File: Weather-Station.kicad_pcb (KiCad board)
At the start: 2 copper layers, 100 x 100 mm, 69 parts, among them J1 PV IN, J10 Lightning Sensor, J11 RG-15 Rain Sensor, J12 BME280 Sensor, J2 TX1, J3 TX2, J4 RX1, J5 RX2, J6 RTD1, J7 RTD2, J8 PDB-C139, J9 TMP36GT9Z, U1 MCP73812T-420I-OT, U2 TPS3700DDCR, U3 TDC1000PW, U4 SiT8918AE-13-33E-5.000000G, U5 TPS73633DBV, U6 TDC7200PW, U7 Wemos_S2, U8 ADS1115IDGS

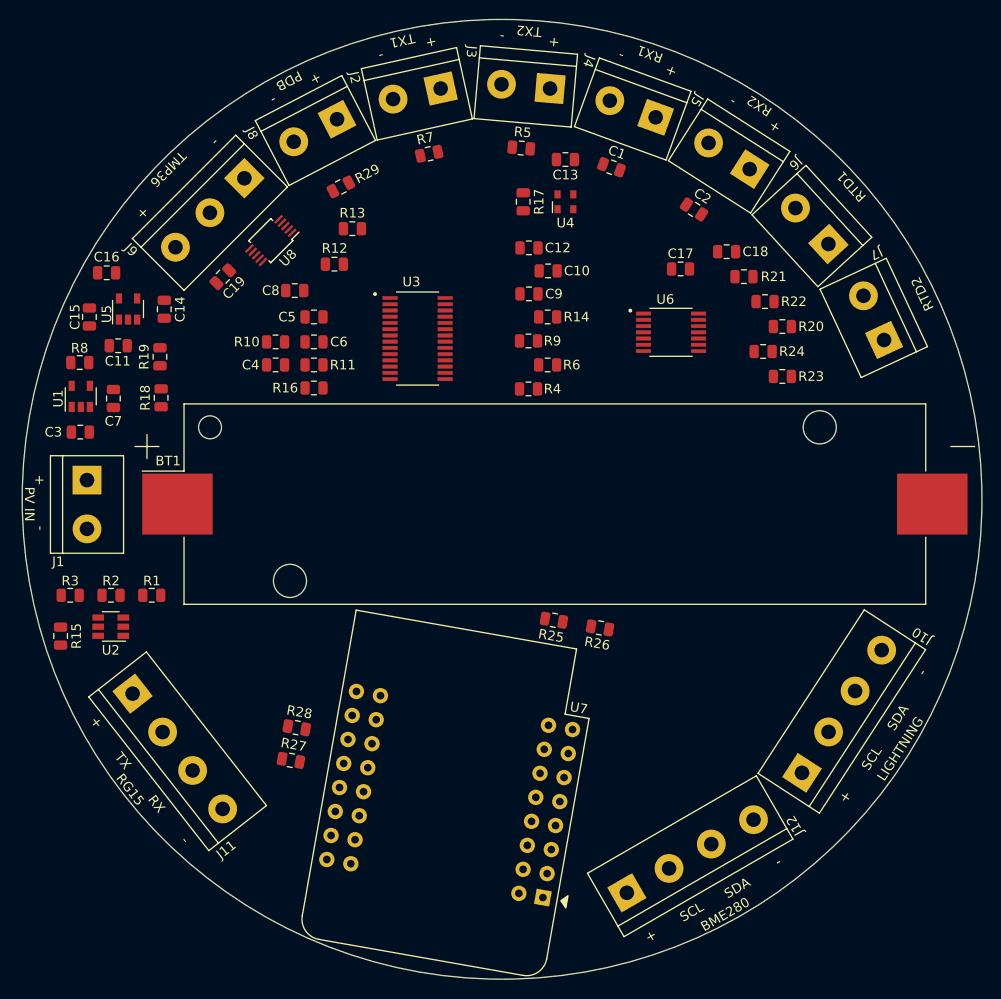
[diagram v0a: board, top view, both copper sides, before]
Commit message: to be continued
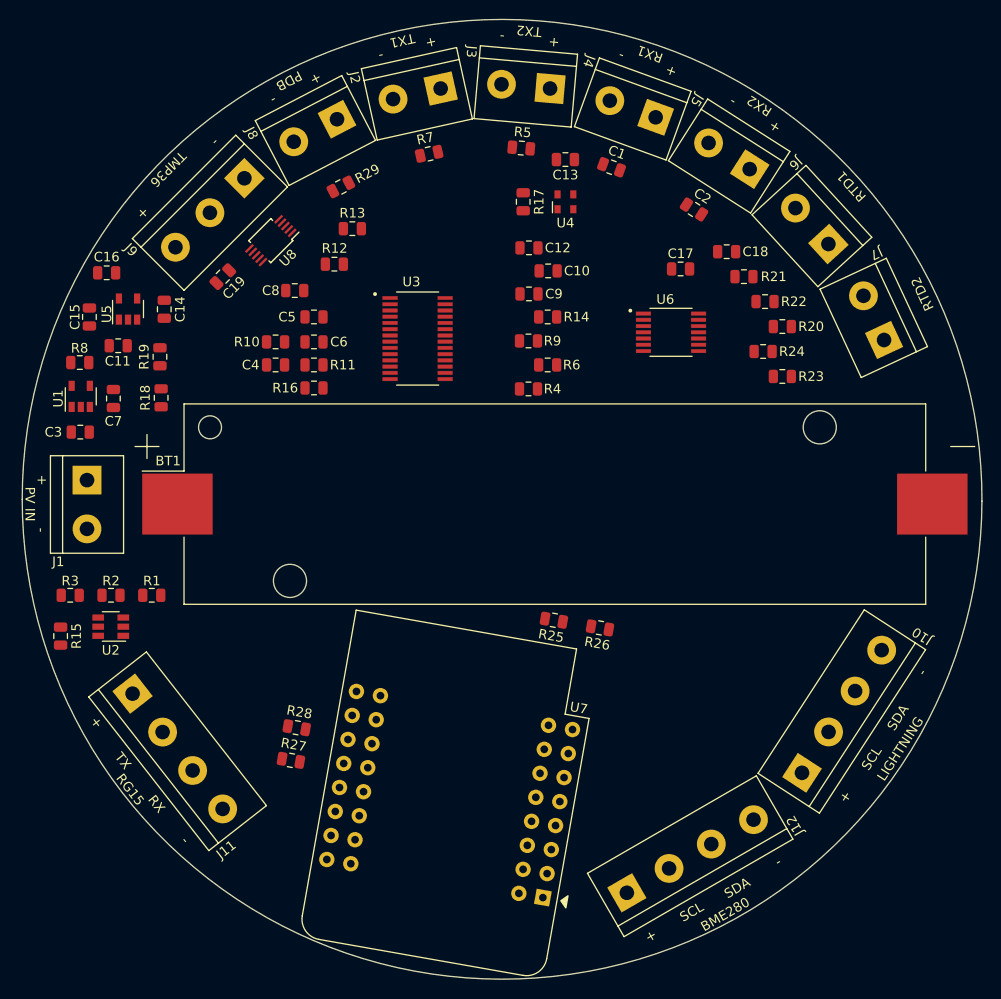
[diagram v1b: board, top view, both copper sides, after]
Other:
- outline, holes or cut-outs redrawn
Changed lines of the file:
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@@
   (general
     (thickness 1.6)
-    (drawings 39)
+    (drawings 40)
     (tracks 0)
     (zones 0)
@@
     )
   )
+  (gr_arc (start 103 94) (end 152.999599 94.199997) (angle -180.2291814) (layer Edge.Cuts) (width 0.05))
+  (gr_arc (start 103 94) (end 53 94) (angle -179.7708181) (layer Edge.Cuts) (width 0.05))
   (gr_text RTD2 (at 146.8 72.6 115) (layer F.SilkS)
     (effects (font (size 1 1) (thickness 0.15)))
@@
     (effects (font (size 1 1) (thickness 0.15)))
   )
-  (gr_text "PV IN" (at 53.75 94.5 270) (layer F.SilkS)
-    (effects (font (size 1 1) (thickness 0.15)))
-  )
-  (gr_text - (at 54.75 97 90) (layer F.SilkS)
-    (effects (font (size 1 1) (thickness 0.15)))
-  )
-  (gr_text + (at 54.75 92 90) (layer F.SilkS)
-    (effects (font (size 1 1) (thickness 0.15)))
-  )
-  (gr_circle (center 103 94) (end 153 94) (layer Edge.Cuts) (width 0.05))
+  (gr_text "PV IN" (at 53.8 94.5 270) (layer F.SilkS)
+    (effects (font (size 1 1) (thickness 0.15)))
+  )
+  (gr_text - (at 54.8 97.2 90) (layer F.SilkS)
+    (effects (font (size 1 1) (thickness 0.15)))
+  )
+  (gr_text + (at 55 92 90) (layer F.SilkS)
+    (effects (font (size 1 1) (thickness 0.15)))
+  )
 )
